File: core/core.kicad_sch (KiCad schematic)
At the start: 68 parts, among them J1 Conn_01x03_Pin, U1 F1C200S, U2 EA3036C, U3 XC6206P302MR_C347375, U4 CH340E, U5 W25Q128JVSIQTR, X1 SMD-3225_4P_24.000MHZ_18PF

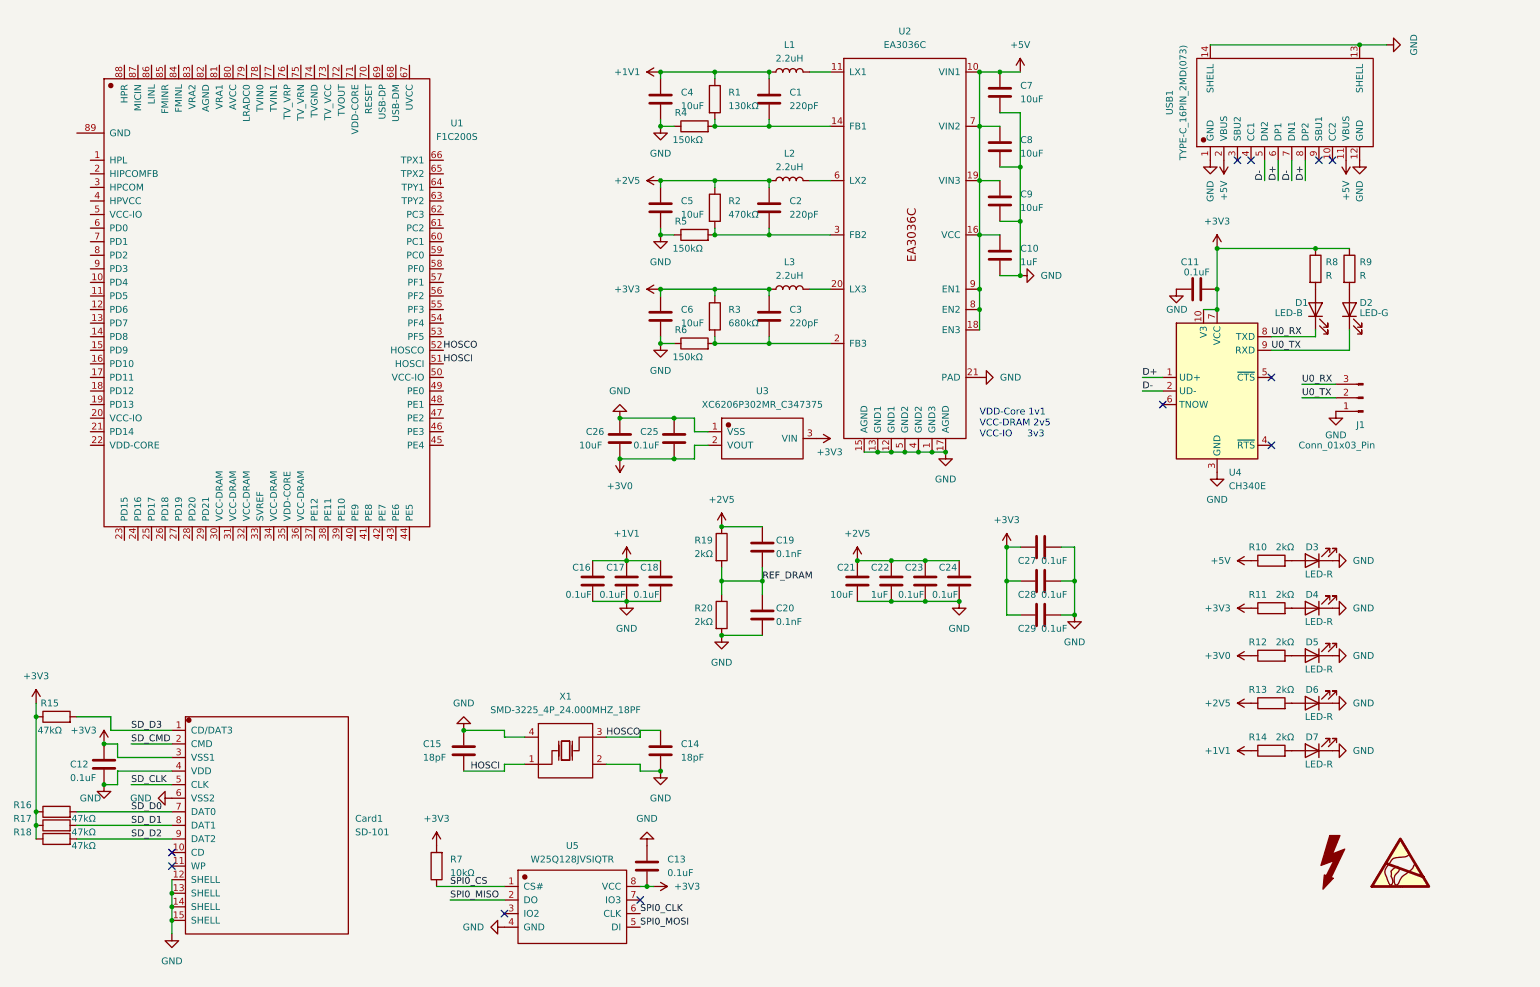
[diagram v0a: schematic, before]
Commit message: finish core schematic
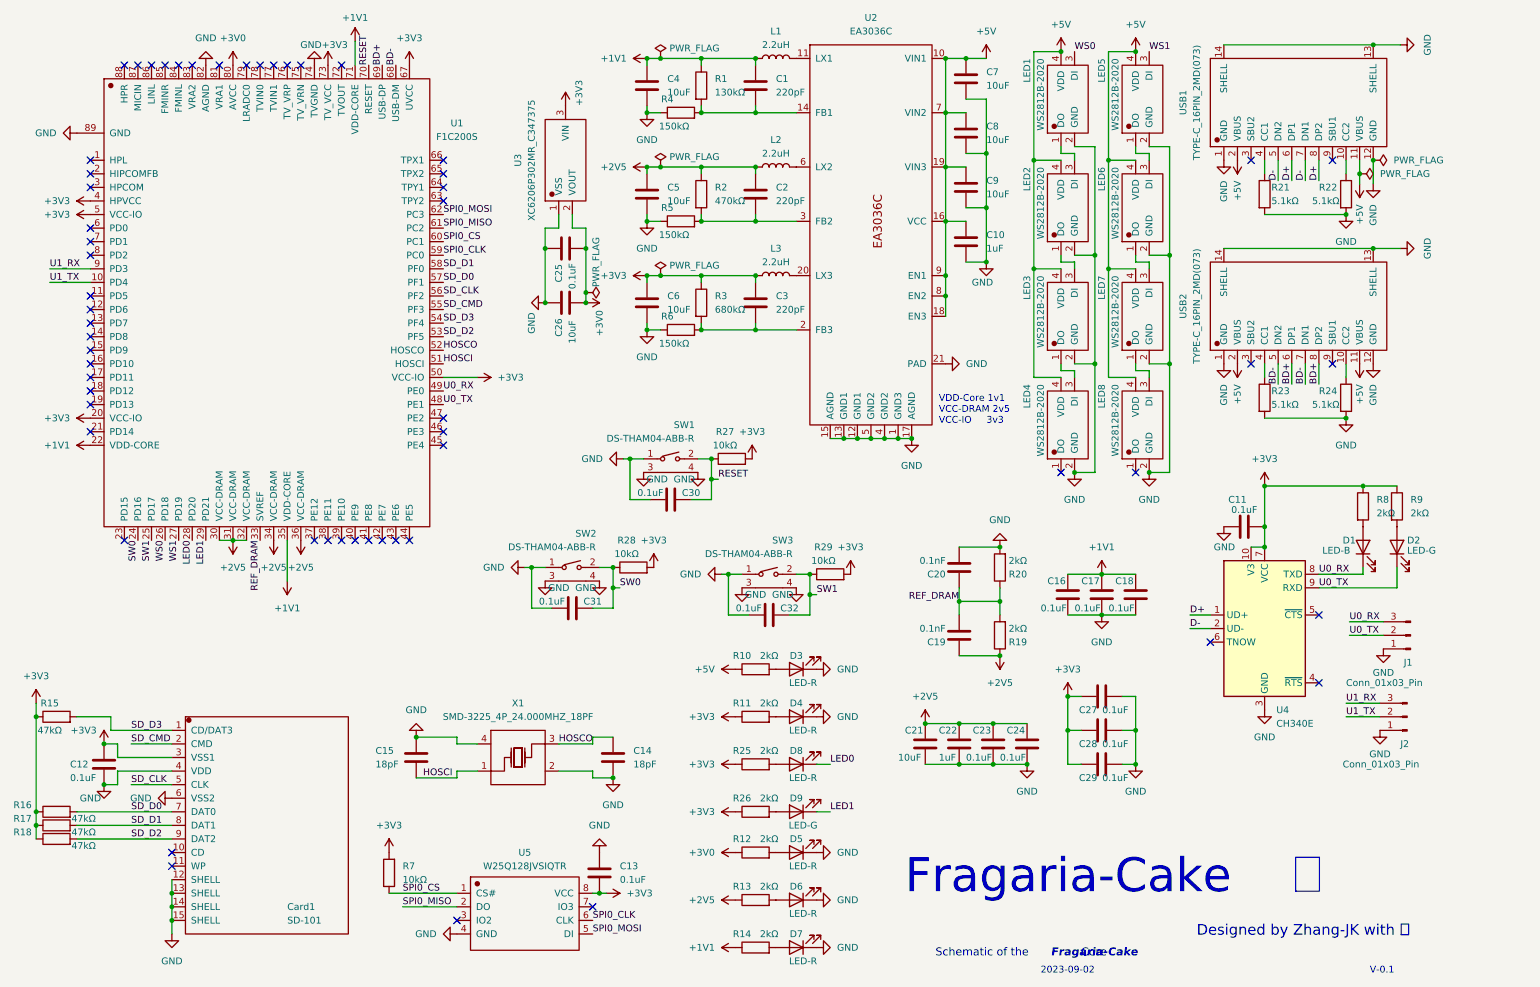
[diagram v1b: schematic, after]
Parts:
- added C30, C31, C32: 0.1uF, Capacitor_SMD:C_0603_1608Metric_Pad1.08x0.95mm_HandSolder, symbol Device:C
- added D8: LED-R, LED_SMD:LED_0603_1608Metric_Pad1.05x0.95mm_HandSolder, symbol Device:LED
- added D9: LED-G, LED_SMD:LED_0603_1608Metric_Pad1.05x0.95mm_HandSolder, symbol Device:LED
- added J2: Conn_01x03_Pin, Connector_PinHeader_1.27mm:PinHeader_1x03_P1.27mm_Vertical, symbol Connector:Conn_01x03_Pin
- added LED1, LED2, LED3, LED4, LED5, LED6, LED7, LED8: WS2812B-2020, kicad_lceda:LED-SMD_4P-L2.0-W2.0-TL_WS2812B-2020, symbol kicad_lceda:WS2812B-2020
- added R21, R22, R23, R24: 5.1kΩ, Resistor_SMD:R_0603_1608Metric_Pad0.98x0.95mm_HandSolder, symbol Device:R
- added R25, R26: 2kΩ, Resistor_SMD:R_0603_1608Metric_Pad0.98x0.95mm_HandSolder, symbol Device:R
- added R27, R28, R29: 10kΩ, Resistor_SMD:R_0603_1608Metric_Pad0.98x0.95mm_HandSolder, symbol Device:R
- added SW1, SW2, SW3: DS-THAM04-ABB-R, kicad_lceda:SW-SMD_D-SWITCH_DS-THAM04-ABB-R, symbol kicad_lceda:DS-THAM04-ABB-R
- added USB2: TYPE-C_16PIN_2MD(073), kicad_lceda:USB-C-SMD_TYPE-C-6PIN-2MD-073, symbol kicad_lceda:TYPE-C_16PIN_2MD(073)
- C10, C11, C12, C13, C14, C15, C7, C8, C9: footprint (none) -> Capacitor_SMD:C_0603_1608Metric_Pad1.08x0.95mm_HandSolder
- C27, C28, C29: footprint Capacitor_SMD:C_0603_1608Metric -> Capacitor_SMD:C_0603_1608Metric_Pad1.08x0.95mm_HandSolder
- J1: footprint Connector_PinHeader_2.54mm:PinHeader_1x03_P2.54mm_Vertical -> Connector_PinHeader_1.27mm:PinHeader_1x03_P1.27mm_Vertical
- R1, R2, R3, R4, R5, R6: footprint Resistor_SMD:R_0201_0603Metric_Pad0.64x0.40mm_HandSolder -> Resistor_SMD:R_0603_1608Metric_Pad0.98x0.95mm_HandSolder
- R10, R11, R12, R13, R14: footprint LED_SMD:LED_0603_1608Metric_Pad1.05x0.95mm_HandSolder -> Resistor_SMD:R_0603_1608Metric_Pad0.98x0.95mm_HandSolder
- R7: footprint (none) -> Resistor_SMD:R_0603_1608Metric_Pad0.98x0.95mm_HandSolder
- R8, R9: value R -> 2kΩ; footprint (none) -> Resistor_SMD:R_0603_1608Metric_Pad0.98x0.95mm_HandSolder
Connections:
- net +1V1: now also U1.22 (VDD-CORE), U1.35 (VDD-CORE), U1.71 (VDD-CORE)
- net +2V5: now also U1.30 (VCC-DRAM), U1.31 (VCC-DRAM), U1.32 (VCC-DRAM), U1.34 (VCC-DRAM), U1.36 (VCC-DRAM)
- net +3V0: now also U1.80 (AVCC)
- net +3V3: now also U1.20 (VCC-IO), U1.4 (HPVCC), U1.5 (VCC-IO), U1.50 (VCC-IO), U1.67 (UVCC), U1.73 (TV_VCC), R25.1, R26.1, R27.2, R28.2, R29.2
- net +5V: now also LED1.4 (VDD), LED2.4 (VDD), LED3.4 (VDD), LED4.4 (VDD), LED5.4 (VDD), LED6.4 (VDD), LED7.4 (VDD), LED8.4 (VDD), USB2.11 (VBUS), USB2.2 (VBUS)
- net GND: now also U1.74 (TVGND), U1.82 (AGND), U1.89 (GND), C30.1, C31.1, C32.1, J2.1 (Pin_1), LED1.2 (GND), LED2.2 (GND), LED3.2 (GND), LED4.2 (GND), LED5.2 (GND), LED6.2 (GND), LED7.2 (GND), LED8.2 (GND), R21.2, R22.2, R23.2, R24.2, SW1.1, SW1.3, SW1.4, SW2.1, SW2.3, SW2.4, SW3.1, SW3.3, SW3.4, USB2.1 (GND), USB2.12 (GND), USB2.13 (SHELL), USB2.14 (SHELL)
- net REF_DRAM: now also U1.33 (SVREF)
- net SD_CLK: now also U1.56 (PF2)
- net SD_CMD: now also U1.55 (PF3)
- net SD_D0: now also U1.57 (PF1)
- net SD_D1: now also U1.58 (PF0)
- net SD_D2: now also U1.53 (PF5)
- net SD_D3: now also U1.54 (PF4)
- net SPI0_CLK: now also U1.59 (PC0)
- net SPI0_CS: now also U1.60 (PC1)
- net SPI0_MISO: now also U1.61 (PC2)
- net SPI0_MOSI: now also U1.62 (PC3)
- net U0_RX: now also U1.49 (PE0)
- net U0_TX: now also U1.48 (PE1)
- net at USB1.10 (CC2): now also R22.1
- net at USB1.4 (CC1): now also R21.1
- net U1_TX: now reaches U1.10 (PD4)
- net U1_TX: now also J2.2 (Pin_2)
- net SW0: now reaches U1.24 (PD16)
- net SW0: now also C31.2, R28.1, SW2.2
- net SW1: now reaches U1.25 (PD17)
- net SW1: now also C32.2, R29.1, SW3.2
- net WS0: now reaches U1.26 (PD18)
- net WS0: now also LED1.3 (DI)
- net WS1: now reaches U1.27 (PD19)
- net WS1: now also LED5.3 (DI)
- net LED0: now reaches U1.28 (PD20)
- net LED0: now also D8.1 (K)
- net LED1: now reaches U1.29 (PD21)
- net LED1: now also D9.1 (K)
- net BD-: now reaches U1.68 (USB-DM)
- net BD-: now also USB2.5 (DN2), USB2.7 (DN1)
- net BD+: now reaches U1.69 (USB-DP)
- net BD+: now also USB2.6 (DP1), USB2.8 (DP2)
- net RESET: now reaches U1.70 (RESET)
- net RESET: now also C30.2, R27.1, SW1.2
- net U1_RX: now reaches U1.9 (PD3)
- net U1_RX: now also J2.3 (Pin_3)
- new net: LED5.1 (DO), LED6.3 (DI)
- new net: LED2.1 (DO), LED3.3 (DI)
- new net: LED1.1 (DO), LED2.3 (DI)
- new net: LED6.1 (DO), LED7.3 (DI)
- new net: LED7.1 (DO), LED8.3 (DI)
- new net: R24.1, USB2.10 (CC2)
- new net: R23.1, USB2.4 (CC1)
- new net: D8.2 (A), R25.2
- new net: D9.2 (A), R26.2
- new net: LED3.1 (DO), LED4.3 (DI)
- no-connect marks 11 -> 58
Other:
- note added: "2023-09-02"
- note added: "Designed by Zhang-JK with 󱢠"
- note added: "Fragaria-Cake"
- note added: "Fragaria-Cake "
- note added: "Schematic of the Core"
- note added: "V-0.1"
- moved on the sheet: C1, C10, C11, C13, C14, C15, C16, C17, C18, C19, C2, C20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
